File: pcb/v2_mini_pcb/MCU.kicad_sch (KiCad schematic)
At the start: 13 parts, among them SW1 SW_Push, SW2 SW_Push

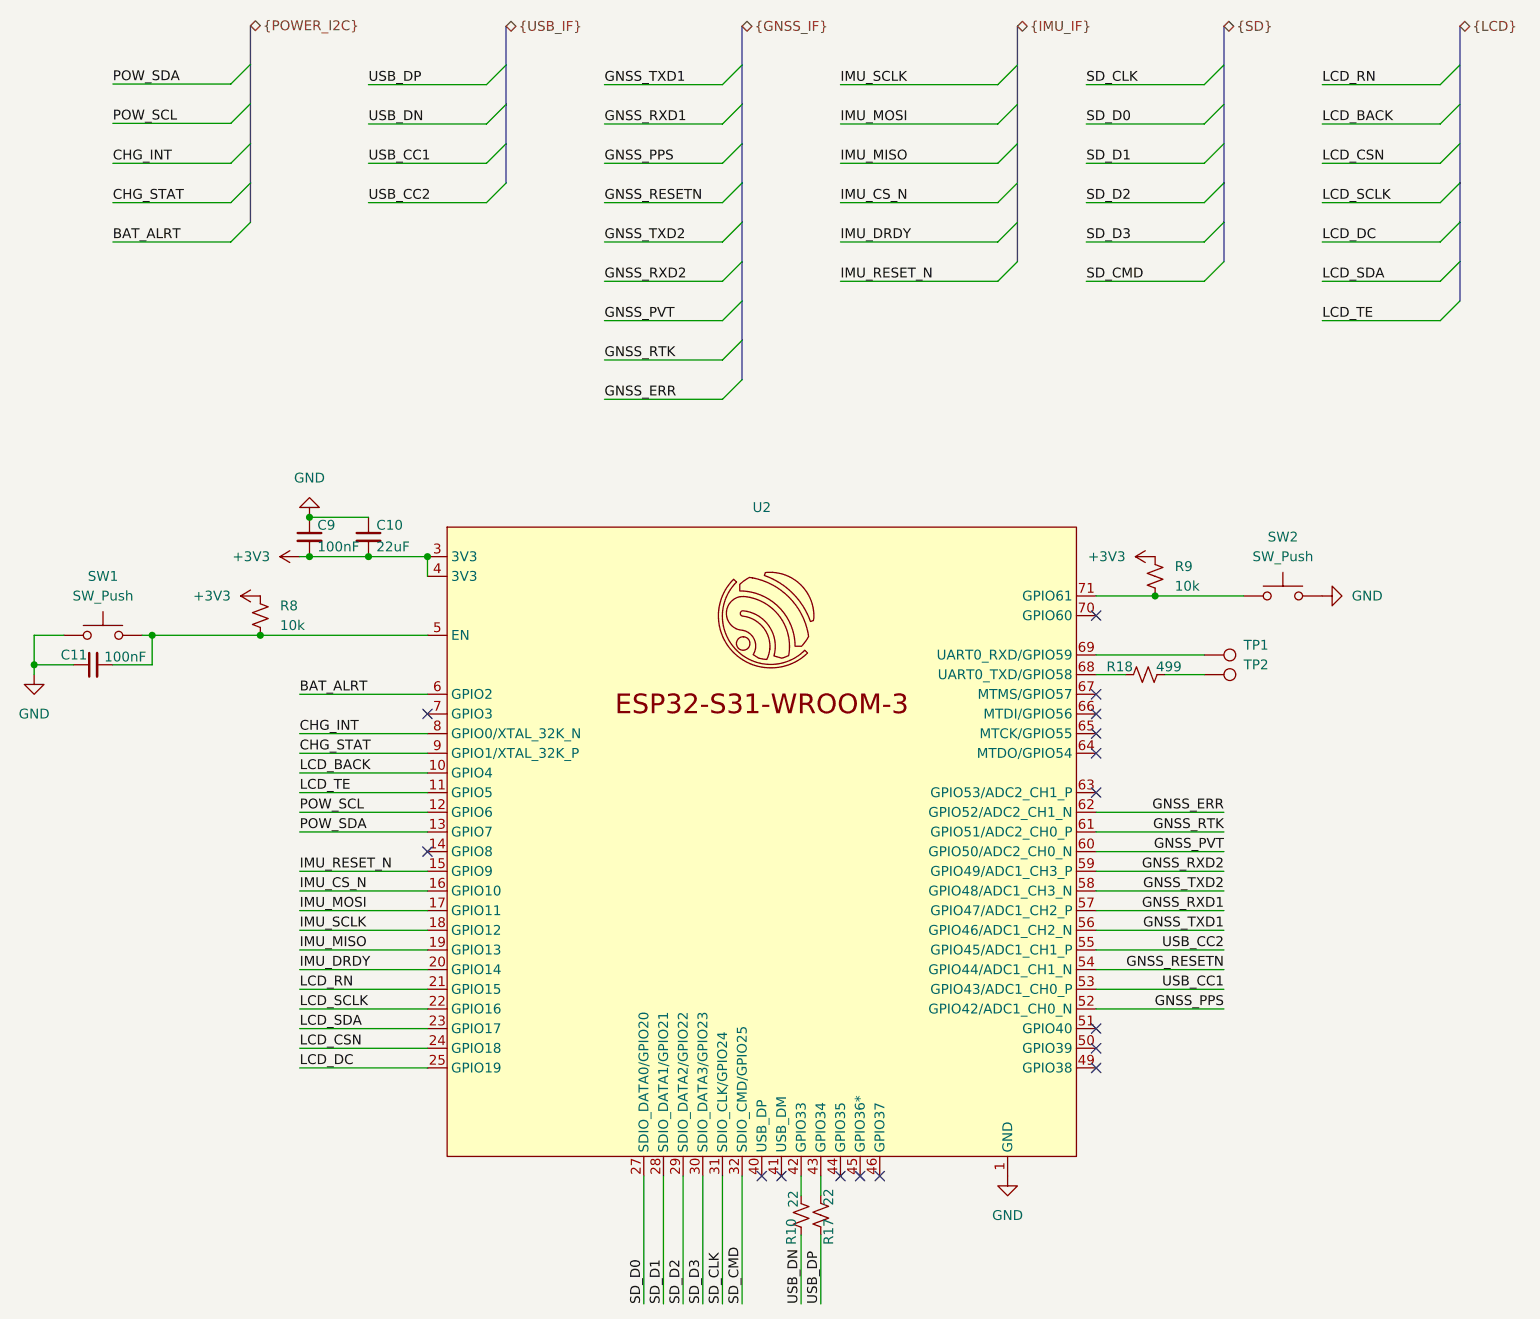
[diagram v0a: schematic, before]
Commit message: erc rules
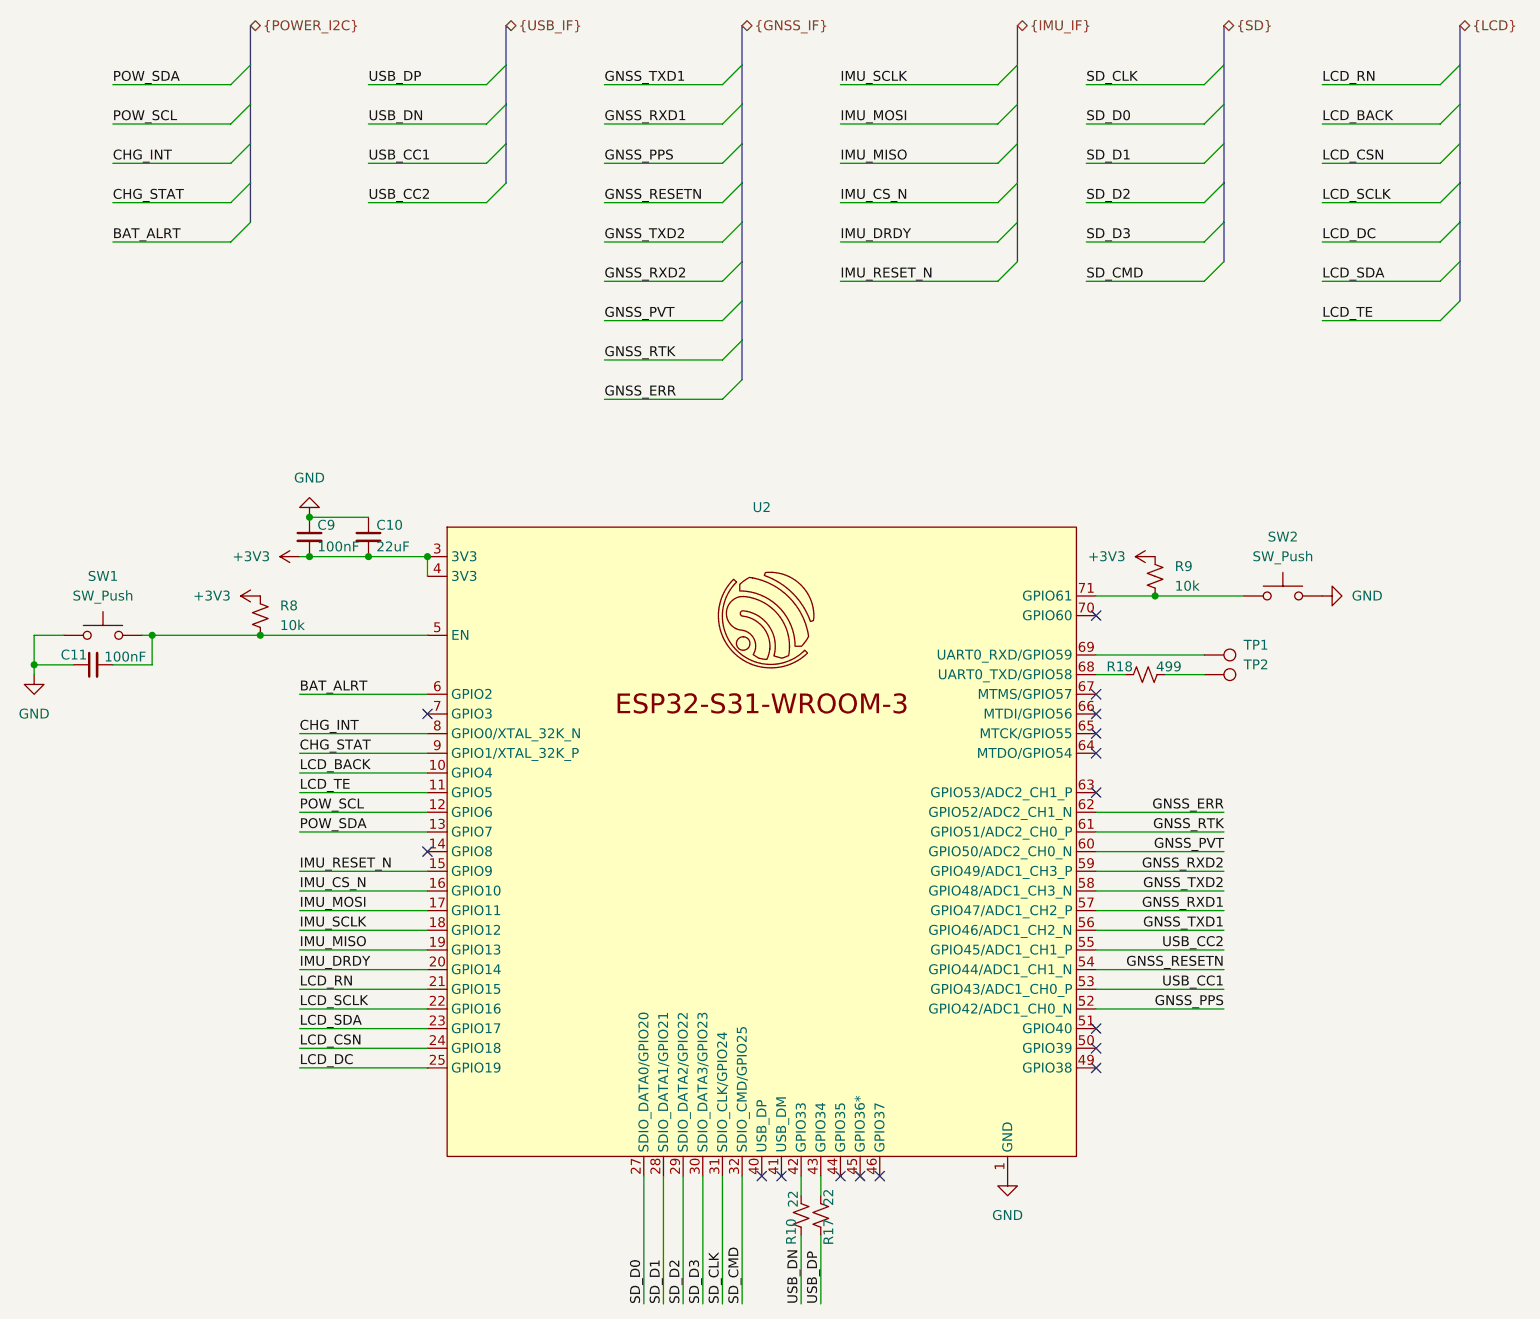
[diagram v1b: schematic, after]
